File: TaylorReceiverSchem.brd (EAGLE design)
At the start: 51.7 x 73.7 mm, 16 parts, among them U1 TEENSY_3.1_BASIC, U2 XBEE_ADAPTER_KIT

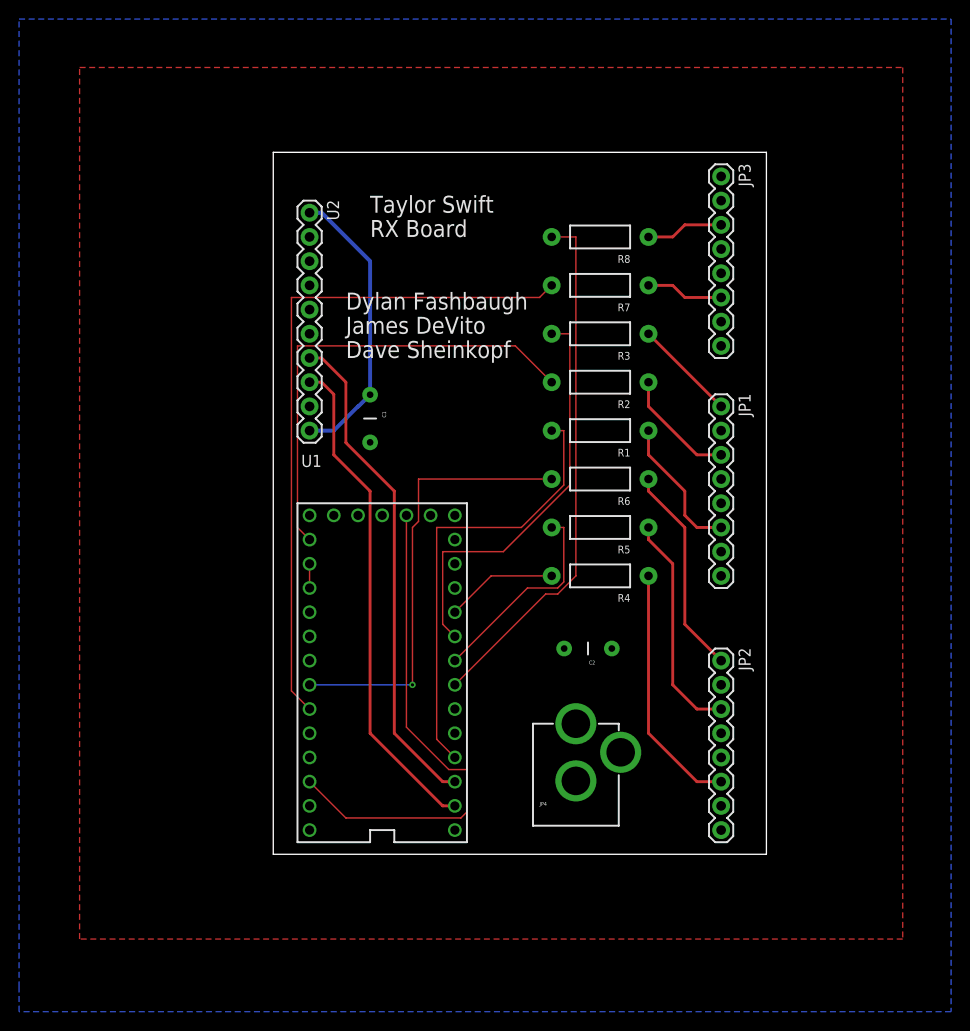
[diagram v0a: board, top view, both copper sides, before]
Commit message: New and improved board design
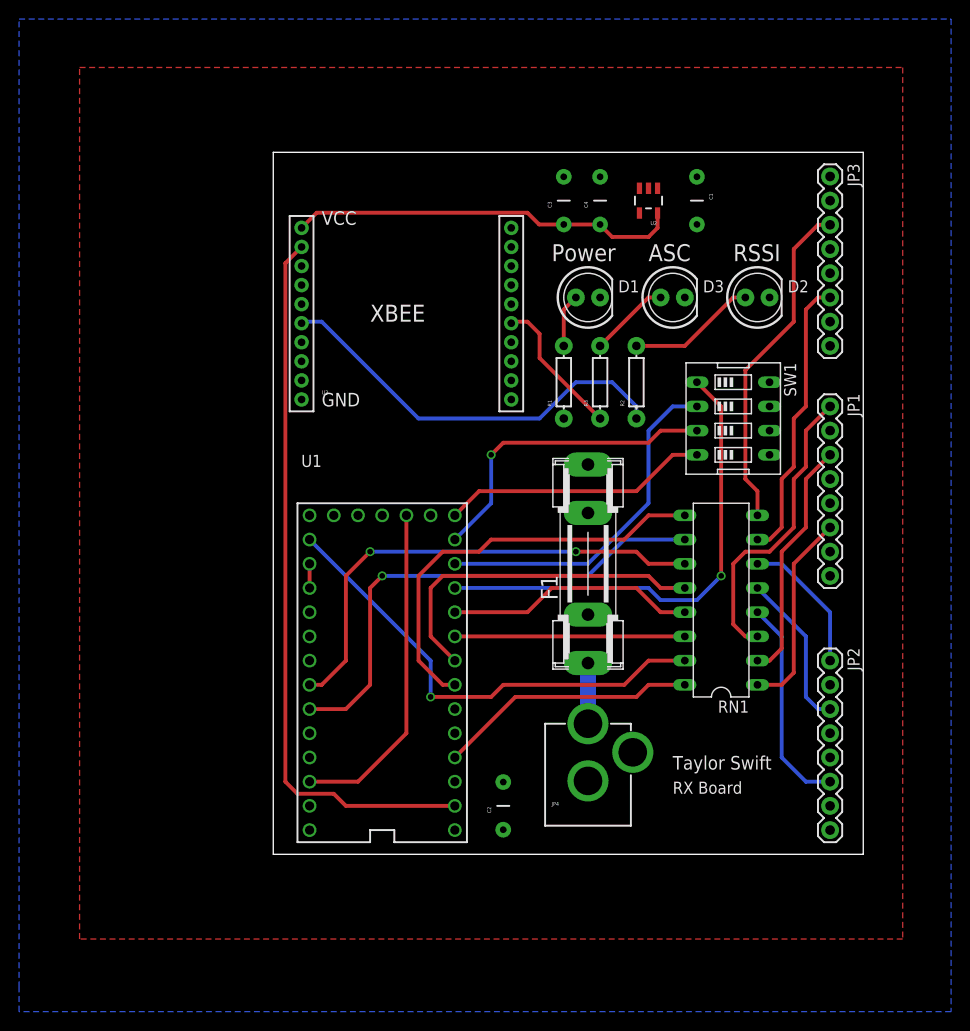
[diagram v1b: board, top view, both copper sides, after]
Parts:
- removed R4, R5, R6, R7, R8: (no value), SparkFun-Resistors:AXIAL-0.4
- added C3, C4: (no value), SparkFun-Capacitors:CAP-PTH-5MM
- added D1, D2, D3: (no value), SparkFun-LED:LED5MM
- added F1: (no value), fuse:SHK20L
- added RN1: (no value), resistor-dil:DIL16
- added SW1: (no value), special:EDG-04
- added U3: XBEE-1B1, SparkFun-RF:XBEE-1
- R1, R2, R3: device SparkFun-Resistors:AXIAL-0.4 -> SparkFun-Passives:AXIAL-0.3
- U2: value XBEE_ADAPTER_KIT -> V_REG_LDOSMD; device Nanotronics:1X10 -> SparkFun-PowerIC:SOT23-5
- moved C1 41.2 mm to (44.5, 68.6)
- moved U2 35.6 mm to (39.4, 68.6), turned to 180 degrees
- moved C2 18.8 mm to (24.1, 5.08), turned to 90 degrees
- moved JP1 11.4 mm to (58.4, 47.0)
- moved JP2 11.4 mm to (58.4, 20.3)
- moved JP3 11.4 mm to (58.4, 71.1)
- moved R1 6.35 mm to (30.5, 49.5), turned to 90 degrees
- moved R3 5.08 mm to (34.3, 49.5), turned to 90 degrees
- moved R2 3.81 mm to (38.1, 49.5), turned to 90 degrees
- moved JP4 1.27 mm to (33.0, 0.00)
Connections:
- removed net N$4: U1.0, U2.8
- removed net N$5: U1.1, U2.7
- new net ASC: R3.P$1, U3.15
- new net DIP1: SW1.1, U1.9
- new net DIP2: SW1.2, U1.10
- new net DIP3: SW1.3, U1.11
- new net DIP4: SW1.4, U1.12
- new net N$15: D1.A, R1.P$2
- new net N$16: D2.A, R2.P$2
- new net N$17: D3.A, R3.P$2
- new net N$2: F1.1A, JP4.PWR
- new net N$3: C3.1, C4.1, U2.5, U3.1
- new net RSSI: R2.P$1, U3.6
- new net XBEERECV: U1.0, U3.2
- net GND: now also C3.2, C4.2, D1.K, D2.K, D3.K, SW1.5, SW1.6, SW1.7, SW1.8, U3.10, U3.3; no longer U2.4
- net N$10: now also RN1.5; no longer R5.P$1
- net N$11: now also RN1.6; no longer R6.P$1
- net N$12: now also RN1.7; no longer R7.P$1
- net N$13: now also RN1.8; no longer R8.P$1
- net N$6: now also RN1.1; no longer R1.P$1
- net N$7: now also RN1.2; no longer R2.P$1
- net N$8: now also RN1.3; no longer R3.P$1
- net N$9: now also RN1.4; no longer R4.P$1
- net STRIP1: now also RN1.16; no longer R1.P$2
- net STRIP2: now also RN1.15; no longer R2.P$2
- net STRIP3: now also RN1.14; no longer R3.P$2
- net STRIP4: now also RN1.13; no longer R4.P$2
- net STRIP5: now also RN1.12; no longer R5.P$2
- net STRIP6: now also RN1.11; no longer R6.P$2
- net STRIP7: now also RN1.10; no longer R7.P$2
- net STRIP8: now also RN1.9; no longer R8.P$2
- net VCC: now also F1.2A, R1.P$1, U2.3; no longer JP4.PWR, U2.10
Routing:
- net XBEERECV: track 0.00 -> 75.6 mm
- net N$4: track 52.3 -> 0.00 mm
- net N$5: track 52.3 -> 0.00 mm
- net DIP1: track 0.00 -> 50.9 mm, vias 0 -> 1
- net RSSI: track 0.00 -> 43.3 mm
- net N$3: track 0.00 -> 41.0 mm
- net DIP2: track 0.00 -> 36.7 mm
- net DIP3: track 0.00 -> 33.1 mm, vias 0 -> 1
- net VCC: track 30.4 -> 0.00 mm
- net DIP4: track 0.00 -> 28.0 mm
- net N$13: track 8.15 -> 35.4 mm
- net N$12: track 8.15 -> 30.0 mm
- net N$8: track 10.8 -> 31.6 mm
- net STRIP1: track 47.1 -> 27.3 mm
- net STRIP3: track 43.4 -> 24.1 mm
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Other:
- board size 51.7 x 73.7 mm -> 61.9 x 73.7 mm
- board text added: "ASC"
- board text added: "Asher Levine"
- board text added: "David Sheinkopf"
- board text added: "GND"
- board text added: "Power"
- board text added: "RSSI"
- board text added: "VCC"
- board text added: "XBEE"
- board text removed: "Dave Sheinkopf"
